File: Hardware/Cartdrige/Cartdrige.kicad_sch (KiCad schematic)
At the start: 5 parts, among them J1 CARTDRIGE, U1 28C256, U2 28C256

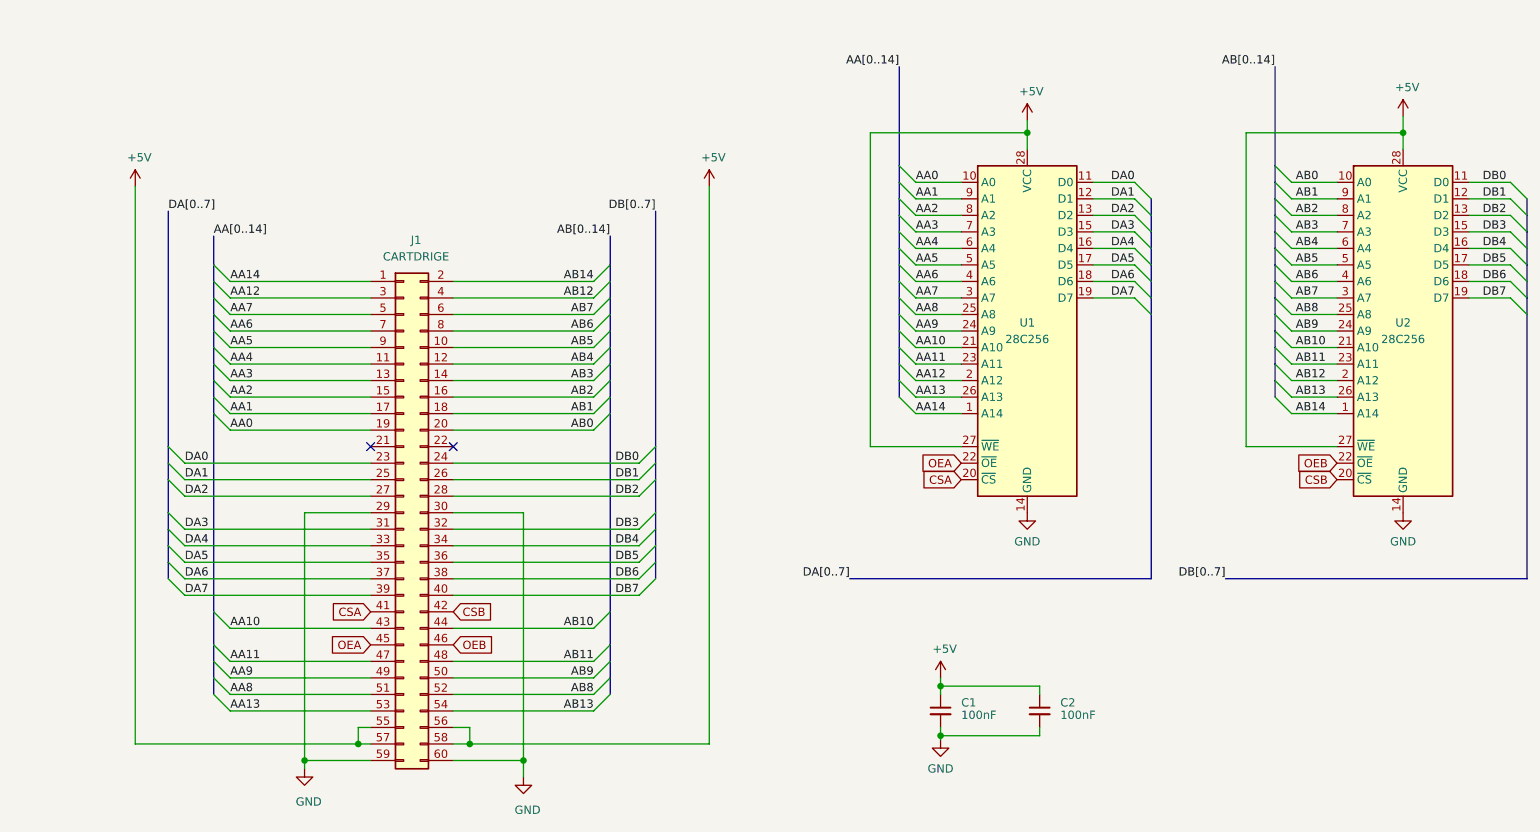
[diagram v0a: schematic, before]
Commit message: Fix
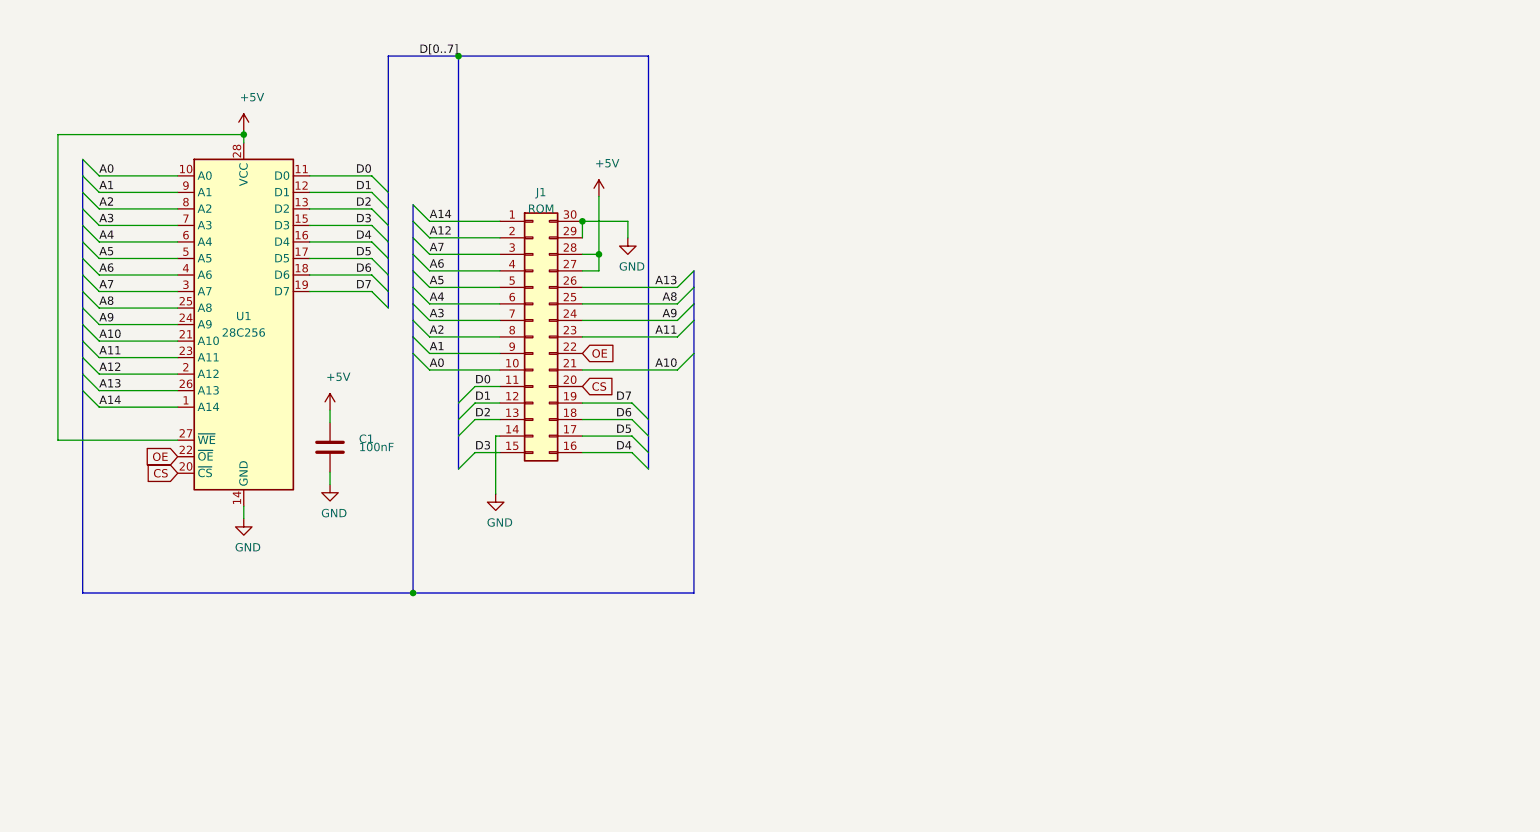
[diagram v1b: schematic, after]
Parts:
- removed C1, C2: 100nF, Capacitor_THT:C_Disc_D5.0mm_W2.5mm_P2.50mm, symbol Device:C_Small
- removed J1: CARTDRIGE, Connector_PCBEdge:Samtec_MECF-30-0_-L-DV_2x30_P1.27mm_Polarized_Edge, symbol Connector_Generic:Conn_02x30_Odd_Even
- removed U2: 28C256, Socket:DIP_Socket-28_W11.9_W12.7_W15.24_W17.78_W18.5_3M_228-1277-00-0602J, symbol Memory_EEPROM:28C256
- added C1: 100nF, Capacitor_THT:C_Disc_D5.0mm_W2.5mm_P2.50mm, symbol Device:C
- added J1: ROM, Connector_TheRLab:NES_PCBEdge, symbol Connector_Generic:Conn_02x15_Counter_Clockwise
- U1: footprint Socket:DIP_Socket-28_W11.9_W12.7_W15.24_W17.78_W18.5_3M_228-1277-00-0602J -> Package_DIP:DIP-28_W15.24mm
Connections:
- net +5V: now also C1.1, J1.27 (Pin_27), J1.28 (Pin_28)
- net GND: now also C1.2, J1.14 (Pin_14), J1.29 (Pin_29), J1.30 (Pin_30)
- net AA0 renamed A0
- net A0: now also J1.10 (Pin_10)
- net AA1 renamed A1
- net A1: now also J1.9 (Pin_9)
- net AA10 renamed A10
- net A10: now also J1.21 (Pin_21)
- net AA11 renamed A11
- net A11: now also J1.23 (Pin_23)
- net AA12 renamed A12
- net A12: now also J1.2 (Pin_2)
- net AA13 renamed A13
- net A13: now also J1.26 (Pin_26)
- net AA14 renamed A14
- net A14: now also J1.1 (Pin_1)
- net AA2 renamed A2
- net A2: now also J1.8 (Pin_8)
- net AA3 renamed A3
- net A3: now also J1.7 (Pin_7)
- net AA4 renamed A4
- net A4: now also J1.6 (Pin_6)
- net AA5 renamed A5
- net A5: now also J1.5 (Pin_5)
- net AA6 renamed A6
- net A6: now also J1.4 (Pin_4)
- net AA7 renamed A7
- net A7: now also J1.3 (Pin_3)
- net AA8 renamed A8
- net A8: now also J1.25 (Pin_25)
- net AA9 renamed A9
- net A9: now also J1.24 (Pin_24)
- net CSA renamed CS
- net CS: now also J1.20 (Pin_20)
- net DA0 renamed D0
- net D0: now also J1.11 (Pin_11)
- net DA1 renamed D1
- net D1: now also J1.12 (Pin_12)
- net DA2 renamed D2
- net D2: now also J1.13 (Pin_13)
- net DA3 renamed D3
- net D3: now also J1.15 (Pin_15)
- net DA4 renamed D4
- net D4: now also J1.16 (Pin_16)
- net DA5 renamed D5
- net D5: now also J1.17 (Pin_17)
- net DA6 renamed D6
- net D6: now also J1.18 (Pin_18)
- net DA7 renamed D7
- net D7: now also J1.19 (Pin_19)
- net OEA renamed OE
- net OE: now also J1.22 (Pin_22)
- no-connect marks 2 -> 0

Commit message: Finalize 1.3
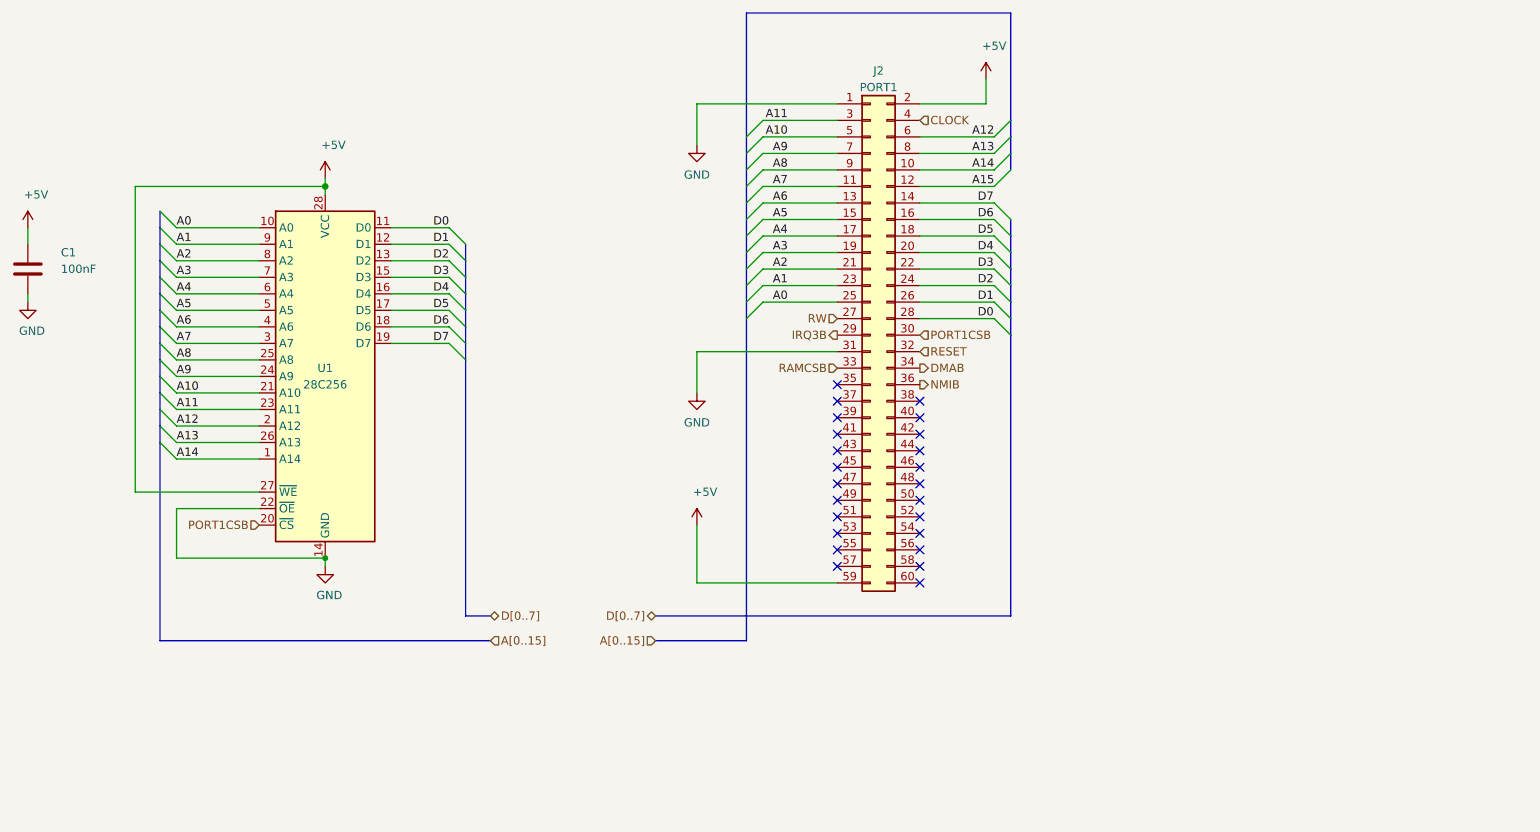
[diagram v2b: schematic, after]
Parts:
- removed J1: ROM, Connector_TheRLab:NES_PCBEdge, symbol Connector_Generic:Conn_02x15_Counter_Clockwise
- added J2: PORT1, NESConnector:NES_PCBEdge, symbol Connector_Generic:Conn_02x30_Odd_Even
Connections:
- net OE is gone; now on net GND: U1.22 (~{OE})
- net +5V: now also J2.2 (Pin_2), J2.59 (Pin_59)
- net A0: now also J2.25 (Pin_25)
- net A1: now also J2.23 (Pin_23)
- net A10: now also J2.5 (Pin_5)
- net A11: now also J2.3 (Pin_3)
- net A12: now also J2.6 (Pin_6)
- net A13: now also J2.8 (Pin_8)
- net A14: now also J2.10 (Pin_10)
- net A2: now also J2.21 (Pin_21)
- net A3: now also J2.19 (Pin_19)
- net A4: now also J2.17 (Pin_17)
- net A5: now also J2.15 (Pin_15)
- net A6: now also J2.13 (Pin_13)
- net A7: now also J2.11 (Pin_11)
- net A8: now also J2.9 (Pin_9)
- net A9: now also J2.7 (Pin_7)
- net D0: now also J2.28 (Pin_28)
- net D1: now also J2.26 (Pin_26)
- net D2: now also J2.24 (Pin_24)
- net D3: now also J2.22 (Pin_22)
- net D4: now also J2.20 (Pin_20)
- net D5: now also J2.18 (Pin_18)
- net D6: now also J2.16 (Pin_16)
- net D7: now also J2.14 (Pin_14)
- net GND: now also J2.1 (Pin_1), J2.31 (Pin_31)
- net CS renamed PORT1CSB
- net PORT1CSB: now also J2.30 (Pin_30)
- new net A15: J2.12 (Pin_12)
- new net CLOCK: J2.4 (Pin_4)
- new net DMAB: J2.34 (Pin_34)
- new net IRQ3B: J2.29 (Pin_29)
- new net NMIB: J2.36 (Pin_36)
- new net RAMCSB: J2.33 (Pin_33)
- new net RESET: J2.32 (Pin_32)
- new net RW: J2.27 (Pin_27)
- no-connect marks 0 -> 24
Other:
- moved on the sheet: C1, U1
